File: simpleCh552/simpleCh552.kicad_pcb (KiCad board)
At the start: 2 copper layers, 27 x 27 mm, 14 parts, among them J1 A0, J2 A1, J3 A2, J4 A3, J5 Conn_01x04, SW1 SW_SPST, U1 CH552G

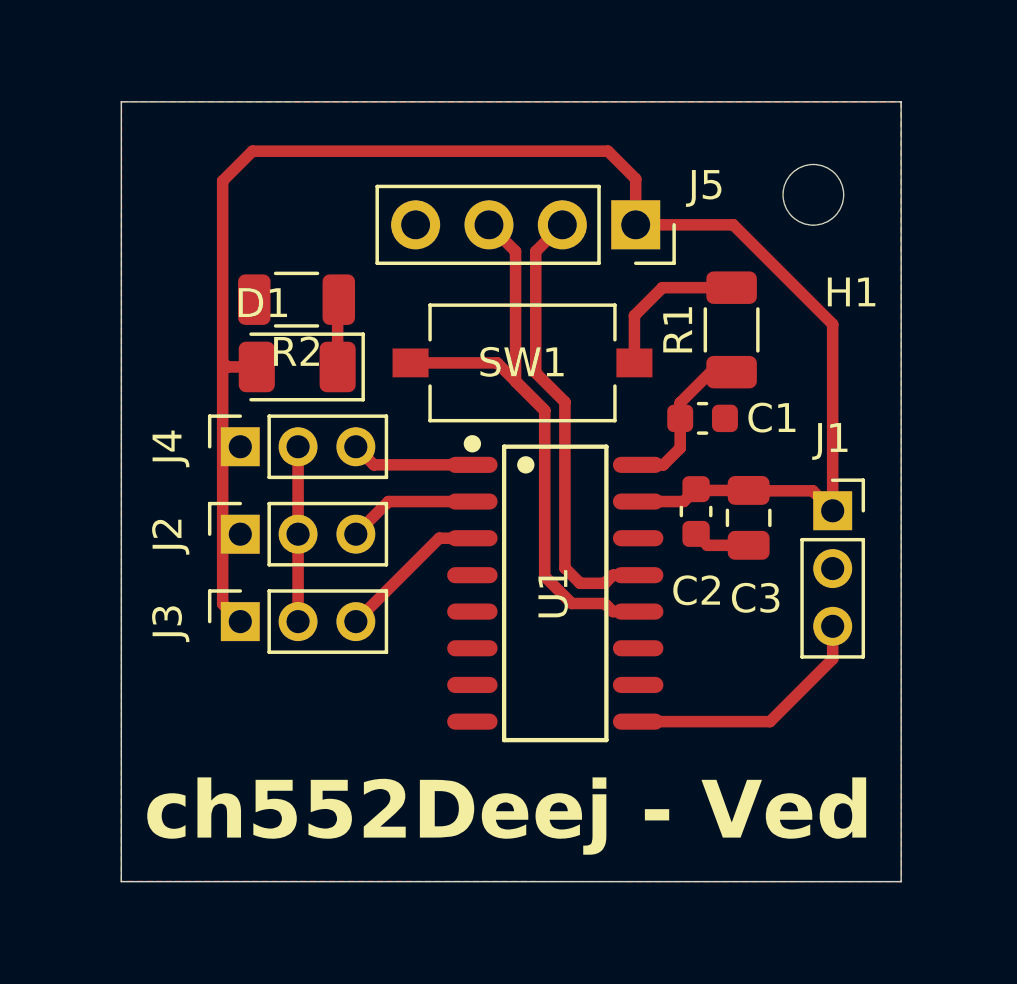
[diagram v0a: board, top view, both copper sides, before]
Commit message: update
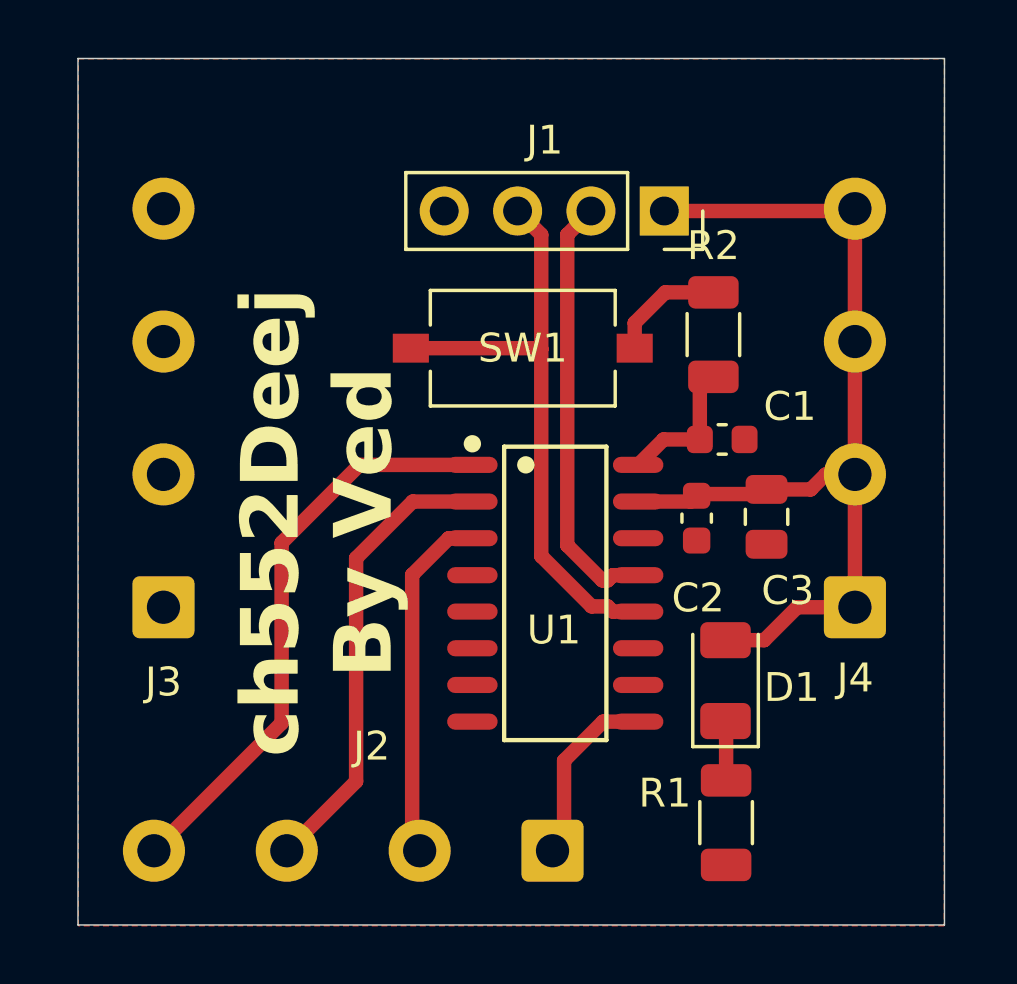
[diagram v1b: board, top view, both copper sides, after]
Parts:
- removed H1: MountingHole, MountingHole:MountingHole_2.1mm
- removed the J1 at (152.7, 62.2)
- J2: value A1 -> Conn_01x04; footprint Connector_PinSocket_2.00mm:PinSocket_1x03_P2.00mm_Vertical -> Connector_Wire:SolderWire-0.5sqmm_1x04_P4.6mm_D0.9mm_OD2.1mm
- J3: value A2 -> Conn_01x04; footprint Connector_PinSocket_2.00mm:PinSocket_1x03_P2.00mm_Vertical -> Connector_Wire:SolderWire-0.5sqmm_1x04_P4.6mm_D0.9mm_OD2.1mm
- J4: value A3 -> Conn_01x04; footprint Connector_PinSocket_2.00mm:PinSocket_1x03_P2.00mm_Vertical -> Connector_Wire:SolderWire-0.5sqmm_1x04_P4.6mm_D0.9mm_OD2.1mm
- moved R1 23.4 mm to (149.0, 73.0), turned to -90 degrees
- moved J4 22.0 mm to (153.5, 65.5)
- moved D1 18.4 mm to (149.0, 68.1), turned to 90 degrees
- moved J2 15.4 mm to (143.0, 74.0), turned to 180 degrees
- moved J3 2.71 mm to (129.6, 65.5)
- moved J1 1.10 mm to (146.9, 51.8)
- moved C1 1.00 mm to (148.9, 59.7)
- moved R2 0.65 mm to (148.6, 56.1)
- moved C3 0.62 mm to (150.4, 62.4)
- moved SW1 0.51 mm to (142.0, 56.6)
- moved C2 0.23 mm to (148.0, 62.5)
- renumbered J5 to J1, R2 to R1, R1 to R2
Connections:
- J2 pad 1: VCC -> A0
- J2 pad 2: GND -> A2
- J3 pad 1: VCC -> GND
- J3 pad 3: A2 -> GND
- J4 pad 2: GND -> VCC
- J4 pad 3: A3 -> VCC
- U1 pad 10: /3.2 -> unconnected-(U1-P3.3/INT1-Pad10)
- U1 pad 11: /3.4 -> unconnected-(U1-P3.4/PWM2/RXD1_/T0-Pad11)
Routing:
- net VCC: track 55.4 -> 33.3 mm
- net A3: track 4.29 -> 20.2 mm
- net A1: track 4.50 -> 16.0 mm
- net GND: track 8.51 -> 0.00 mm
- net A2: track 5.23 -> 12.3 mm
- net A0: track 8.76 -> 6.64 mm
- net Net-(SW1-B): track 5.40 -> 3.79 mm
- net /D+: track 22.0 -> 21.0 mm
- net /D-: track 15.6 -> 14.9 mm
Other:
- board size 27 x 27 mm -> 30 x 30 mm
- board text added: "ch552Deej By Ved"
- board text removed: "ch552Deej - Ved"
